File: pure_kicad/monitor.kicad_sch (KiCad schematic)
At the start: 46 parts, among them J3 XT60M, J4 XT60M, J5 Conn_01x04_Pin, J6 Conn_01x04_Pin, Q5 Q_PMOS_SGD, Q6 Q_NMOS_DGS, Q7 Q_NMOS_DGS, U2 BQ40Z80RSMR

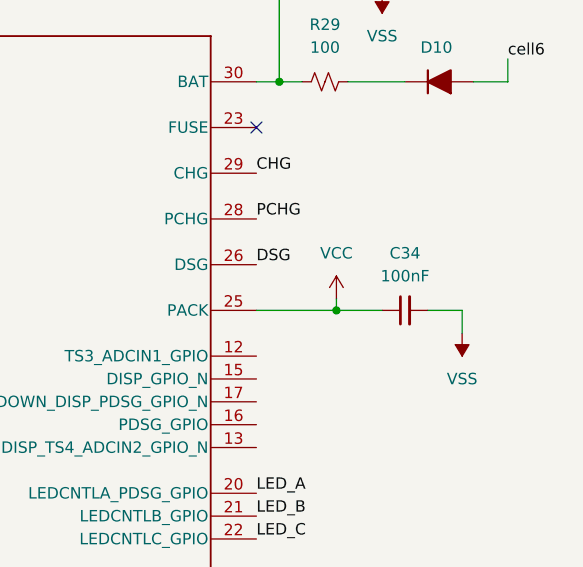
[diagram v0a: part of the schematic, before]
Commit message: I think this was just sorting LEDs
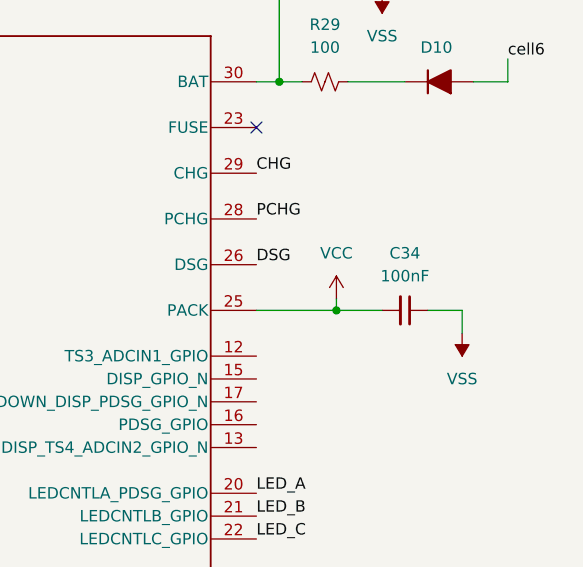
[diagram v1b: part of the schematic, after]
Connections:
- net -BATT: now also C34.1; no longer C34.2
- net VCC: now also C34.2; no longer C34.1
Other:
- moved on the sheet: C34
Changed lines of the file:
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@@
 	(symbol
 		(lib_id "Device:C_Small")
-		(at 217.17 99.06 90)
+		(at 217.17 99.06 270)
+		(mirror x)
 		(unit 1)
 		(exclude_from_sim no)
@@
 		(on_board yes)
 		(dnp no)
-		(fields_autoplaced yes)
 		(property "Reference" "C34"
-			(at 217.1763 92.71 90)
+			(at 217.1637 92.71 90)
 			(effects
 				(font
@@
 		)
 		(property "Value" "100nF"
-			(at 217.1763 95.25 90)
+			(at 217.1637 95.25 90)
 			(effects
 				(font
